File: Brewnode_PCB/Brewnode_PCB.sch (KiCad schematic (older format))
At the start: 0 parts

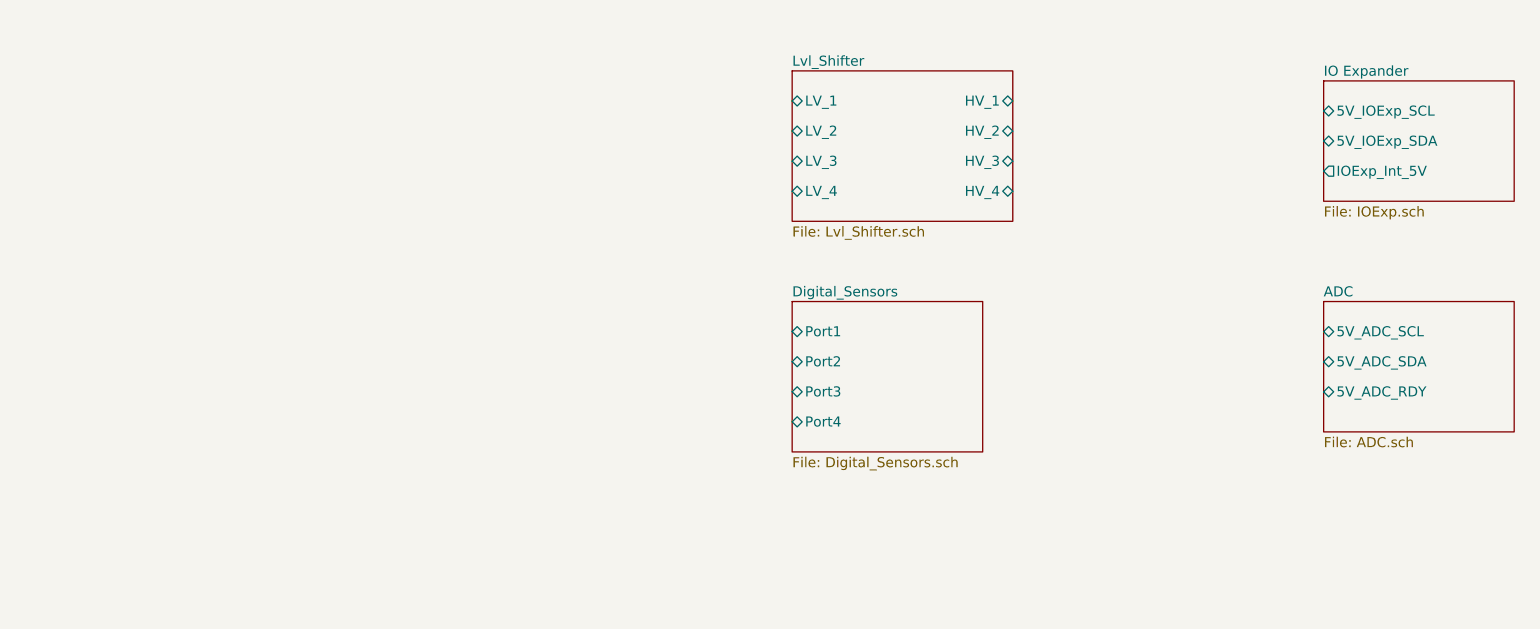
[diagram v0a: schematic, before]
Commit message: More PCB Sch work
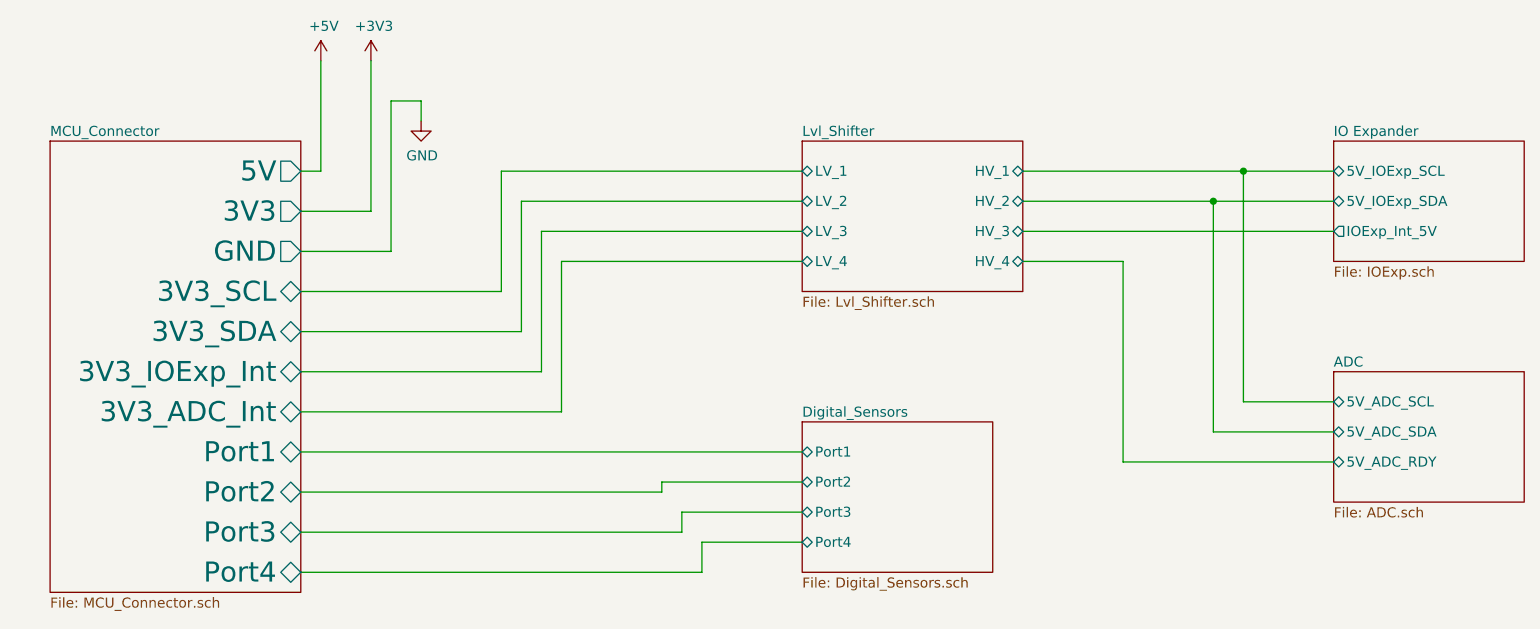
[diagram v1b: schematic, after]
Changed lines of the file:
@@
 $Descr A4 11693 8268
 encoding utf-8
-Sheet 1 7
+Sheet 1 8
 Title "BrewnodeV1"
-Date "2020-09-15"
+Date "2020-09-16"
 Rev "1.0"
 Comp "Halldin"
@@
 $EndDescr
 $Sheet
-S 9000 1100 950  600
+S 9050 1400 950  600
 U 5F5F1150
 F0 "IO Expander" 50
 F1 "IOExp.sch" 50
-F2 "IOExp_Int_5V" O L 9000 1550 50
-F3 "5V_IOExp_SDA" B L 9000 1400 50
-F4 "5V_IOExp_SCL" B L 9000 1250 50
+F2 "IOExp_Int_5V" O L 9050 1850 50
+F3 "5V_IOExp_SDA" B L 9050 1700 50
+F4 "5V_IOExp_SCL" B L 9050 1550 50
 $EndSheet
 $Sheet
-S 9000 2200 950  650
+S 9050 2550 950  650
 U 5F66CC9A
 F0 "ADC" 50
 F1 "ADC.sch" 50
-F2 "5V_ADC_SCL" B L 9000 2350 50
-F3 "5V_ADC_SDA" B L 9000 2500 50
-F4 "5V_ADC_RDY" B L 9000 2650 50
+F2 "5V_ADC_SCL" B L 9050 2700 50
+F3 "5V_ADC_SDA" B L 9050 2850 50
+F4 "5V_ADC_RDY" B L 9050 3000 50
 $EndSheet
 $Sheet
-S 6350 1050 1100 750
+S 6400 1400 1100 750
 U 5F6162C4
 F0 "Lvl_Shifter" 50
 F1 "Lvl_Shifter.sch" 50
-F2 "LV_1" B L 6350 1200 50
-F3 "LV_2" B L 6350 1350 50
-F4 "LV_3" B L 6350 1500 50
-F5 "LV_4" B L 6350 1650 50
-F6 "HV_1" B R 7450 1200 50
-F7 "HV_2" B R 7450 1350 50
-F8 "HV_3" B R 7450 1500 50
-F9 "HV_4" B R 7450 1650 50
+F2 "LV_1" B L 6400 1550 50
+F3 "LV_2" B L 6400 1700 50
+F4 "LV_3" B L 6400 1850 50
+F5 "LV_4" B L 6400 2000 50
+F6 "HV_1" B R 7500 1550 50
+F7 "HV_2" B R 7500 1700 50
+F8 "HV_3" B R 7500 1850 50
+F9 "HV_4" B R 7500 2000 50
 $EndSheet
 $Sheet
-S 6350 2200 950  750
+S 6400 2800 950  750
 U 5F66FC6A
 F0 "Digital_Sensors" 50
 F1 "Digital_Sensors.sch" 50
-F2 "Port1" B L 6350 2350 50
-F3 "Port2" B L 6350 2500 50
-F4 "Port3" B L 6350 2650 50
-F5 "Port4" B L 6350 2800 50
+F2 "Port1" B L 6400 2950 50
+F3 "Port2" B L 6400 3100 50
+F4 "Port3" B L 6400 3250 50
+F5 "Port4" B L 6400 3400 50
 $EndSheet
+$Sheet
+S 2650 1400 1250 2250
+U 5F61AF49
+F0 "MCU_Connector" 50
+F1 "MCU_Connector.sch" 50
+F2 "5V" O R 3900 1550 100
+F3 "3V3" O R 3900 1750 100
+F4 "GND" O R 3900 1950 100
+F5 "Port1" B R 3900 2950 100
+F6 "Port2" B R 3900 3150 100
+F7 "Port3" B R 3900 3350 100
+F8 "Port4" B R 3900 3550 100
+F9 "3V3_SCL" B R 3900 2150 100
+F10 "3V3_SDA" B R 3900 2350 100
+F11 "3V3_IOExp_Int" B R 3900 2550 100
+F12 "3V3_ADC_Int" B R 3900 2750 100
+$EndSheet
+$Comp
+L power:+3V3 #PWR?
+U 1 1 5F6234F7
+P 4250 1000
+F 0 "#PWR?" H 4250 850 50  0001 C CNN
+F 1 "+3V3" H 4265 1173 50  0000 C CNN
+F 2 "" H 4250 1000 50  0001 C CNN
+F 3 "" H 4250 1000 50  0001 C CNN
+	1    4250 1000
+	1    0    0    -1
+$EndComp
+$Comp
+L power:+5V #PWR?
+U 1 1 5F6241F4
+P 4000 1000
+F 0 "#PWR?" H 4000 850 50  0001 C CNN
+F 1 "+5V" H 4015 1173 50  0000 C CNN
+F 2 "" H 4000 1000 50  0001 C CNN
+F 3 "" H 4000 1000 50  0001 C CNN
+	1    4000 1000
+	1    0    0    -1
+$EndComp
+$Comp
+L power:GND #PWR?
+U 1 1 5F6246CE
+P 4500 1300
+F 0 "#PWR?" H 4500 1050 50  0001 C CNN
+F 1 "GND" H 4505 1127 50  0000 C CNN
+F 2 "" H 4500 1300 50  0001 C CNN
+F 3 "" H 4500 1300 50  0001 C CNN
+	1    4500 1300
+	1    0    0    -1
+$EndComp
+Wire Wire Line
+	3900 1550 4000 1550
+Wire Wire Line
+	4000 1550 4000 1000
+Wire Wire Line
+	3900 1750 4250 1750
+Wire Wire Line
+	4250 1750 4250 1000
+Wire Wire Line
+	3900 1950 4350 1950
+Wire Wire Line
+	4350 1950 4350 1200
+Wire Wire Line
+	4350 1200 4500 1200
+Wire Wire Line
+	4500 1200 4500 1300
+Wire Wire Line
+	3900 2150 4900 2150
+Wire Wire Line
+	4900 2150 4900 1550
+Wire Wire Line
+	4900 1550 6400 1550
+Wire Wire Line
+	3900 2350 5000 2350
+Wire Wire Line
+	5000 2350 5000 1700
+Wire Wire Line
+	5000 1700 6400 1700
+Wire Wire Line
+	3900 2550 5100 2550
+Wire Wire Line
+	5100 2550 5100 1850
+Wire Wire Line
+	5100 1850 6400 1850
+Wire Wire Line
+	3900 2750 5200 2750
+Wire Wire Line
+	5200 2750 5200 2000
+Wire Wire Line
+	5200 2000 6400 2000
+Wire Wire Line
+	3900 3350 5800 3350
+Wire Wire Line
+	5800 3350 5800 3250
+Wire Wire Line
+	5800 3250 6400 3250
+Wire Wire Line
+	3900 3550 5900 3550
+Wire Wire Line
+	5900 3550 5900 3400
+Wire Wire Line
+	5900 3400 6400 3400
+Wire Wire Line
+	7500 2000 8000 2000
+Wire Wire Line
+	8000 2000 8000 3000
+Wire Wire Line
+	8000 3000 9050 3000
+Wire Wire Line
+	7500 1550 8600 1550
+Wire Wire Line
+	7500 1700 8450 1700
+Wire Wire Line
+	9050 1850 7500 1850
+Wire Wire Line
+	9050 2700 8600 2700
+Wire Wire Line
+	8600 2700 8600 1550
+Connection ~ 8600 1550
+Wire Wire Line
+	8600 1550 9050 1550
+Wire Wire Line
+	9050 2850 8450 2850
+Wire Wire Line
+	8450 2850 8450 1700
+Connection ~ 8450 1700
+Wire Wire Line
+	8450 1700 9050 1700
+Wire Wire Line
+	3900 3150 5700 3150
+Wire Wire Line
+	3900 2950 6400 2950
+Wire Wire Line
+	5700 3100 6400 3100
+Wire Wire Line
+	5700 3150 5700 3100
 $EndSCHEMATC
